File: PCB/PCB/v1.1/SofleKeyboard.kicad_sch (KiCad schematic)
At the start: 126 parts

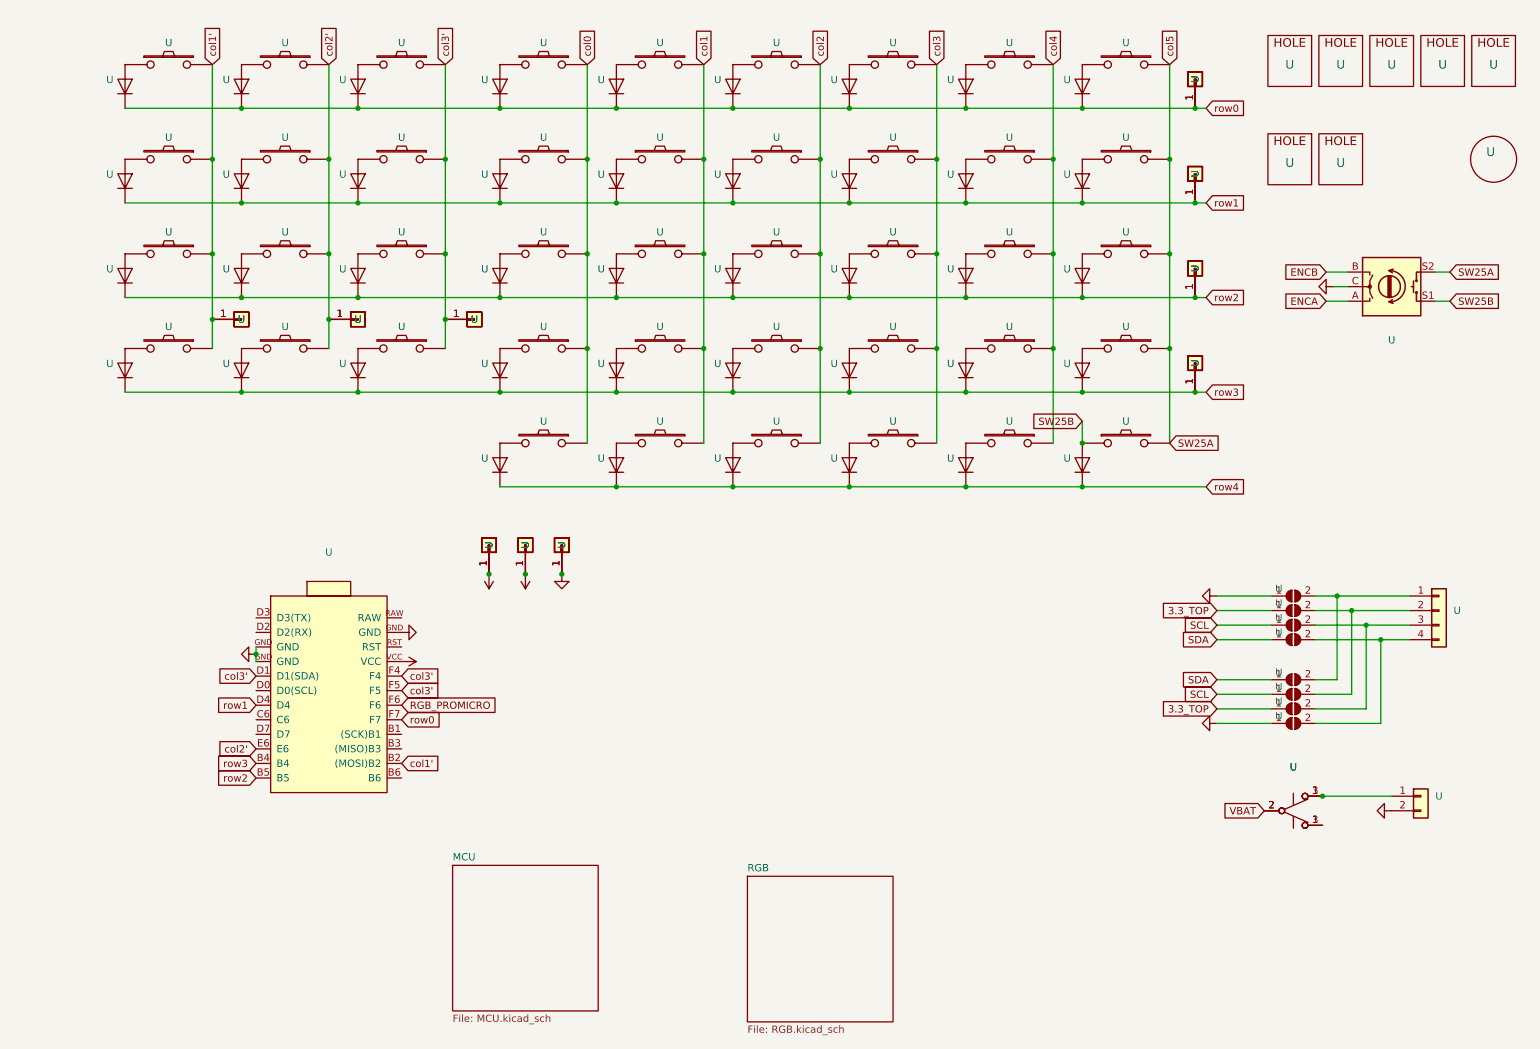
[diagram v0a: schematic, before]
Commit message: update PCB file
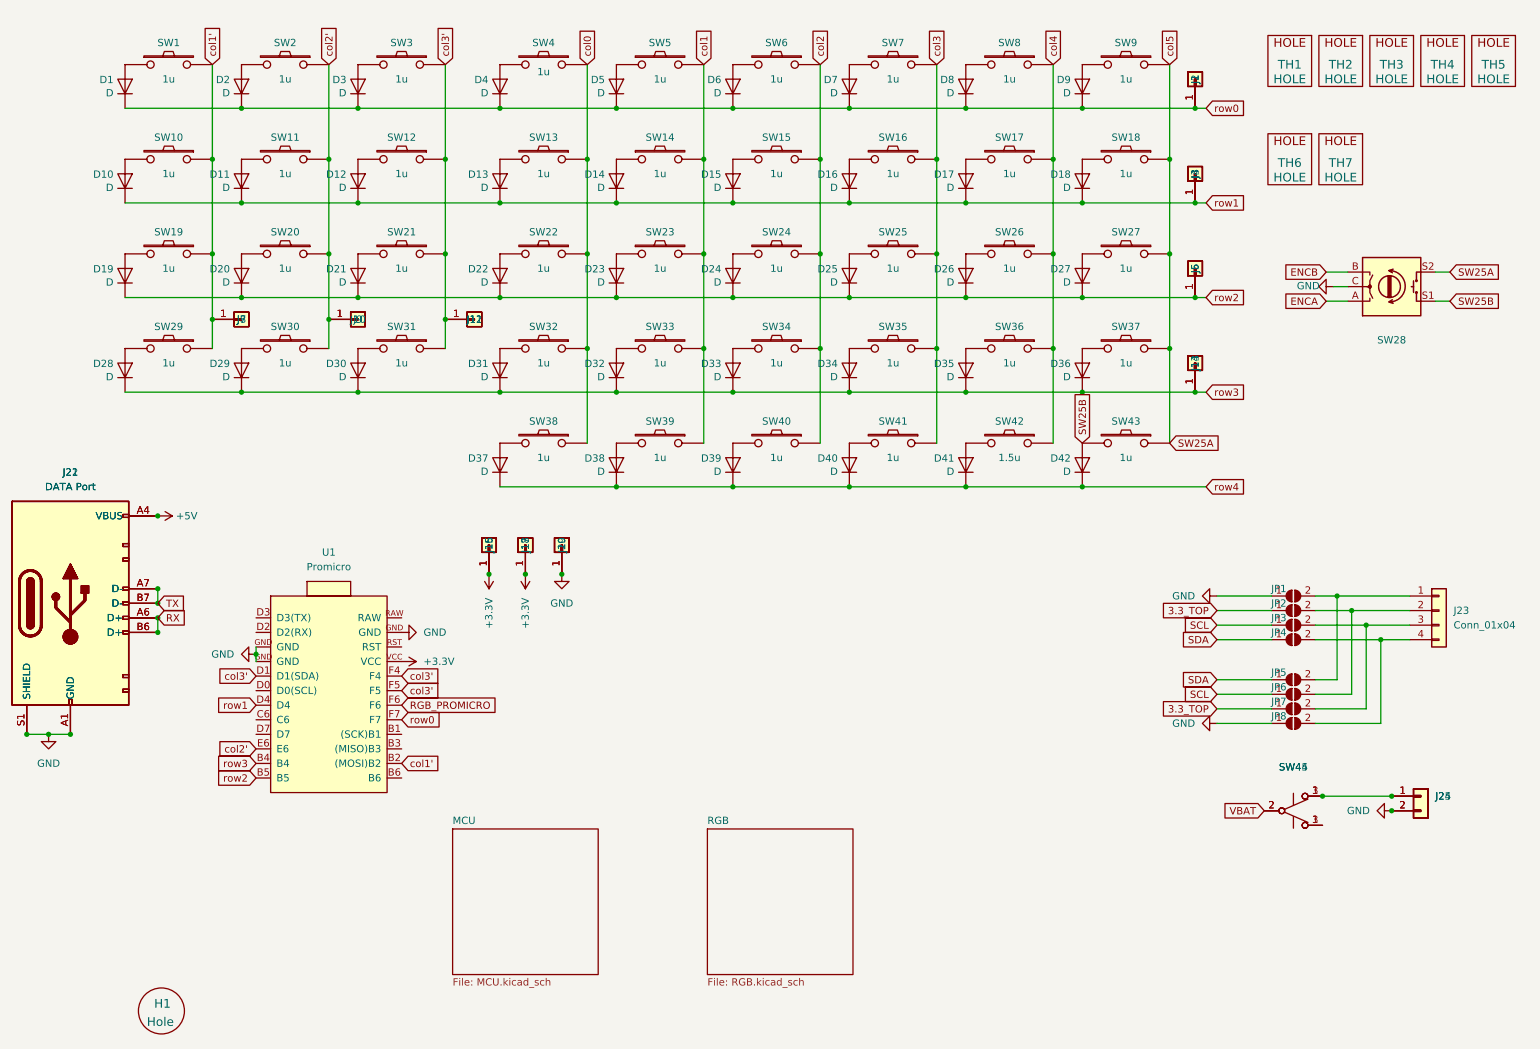
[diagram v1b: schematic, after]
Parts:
- removed U: (no value), symbol SofleKeyboard-rescue:SW_PUSH-Lily58-cache-Lily58_Pro-rescue
- added J21, J22: DATA Port, kien242:USB-C-16pin-hight-v2, symbol Connector:USB_C_Receptacle_USB2.0
- added J24: (no value), kien242:JST_PH_S2B-PH-SM4-TB_1x02-1MP_P2.00mm_Horizontal, symbol Connector_Generic:Conn_01x02
- added SW43: 1u, Library:SW-HS_flip-1u, symbol SofleKeyboard-rescue:SW_PUSH-Lily58-cache-Lily58_Pro-rescue
- D1, D10, D11, D12, D13, D14, D15, D16, D17, D18, D19, D2, D20, D21, D22, D23, D24, D25, D26, D27, D28, D29, D3, D30, D31, D32, D33, D34, D35, D36, D37, D38, D39, D4, D40, D41, D42, D5, D6, D7, D8, D9: renamed from U; value (none) -> D; footprint (none) -> Library:Diode
- H1: renamed from U; value (none) -> Hole; footprint (none) -> Library:Cut_hole
- J1, J10, J11, J12, J13, J14, J15, J16, J17, J18, J19, J2, J20, J3, J4, J5, J6, J7, J8, J9: renamed from U; value (none) -> (none); footprint (none) -> Library:Conn_01x01
- J23: renamed from U; value (none) -> Conn_01x04; footprint (none) -> kien242:128x64OLED
- J25: renamed from U; value (none) -> (none); footprint (none) -> kien242:JST_PH_S2B-PH-SM4-TB_1x02-1MP_P2.00mm_Horizontal
- JP1, JP2, JP3, JP4: renamed from U; value (none) -> (none); footprint (none) -> Jumper:SolderJumper-2_P1.3mm_Open_RoundedPad1.0x1.5mm
- JP5, JP6, JP7, JP8: renamed from U; value (none) -> (none); footprint (none) -> Jumper:SolderJumper-2_P1.3mm_Open_Pad1.0x1.5mm
- SW1, SW10, SW13, SW14, SW15, SW16, SW17, SW18, SW19, SW2, SW20, SW21, SW22, SW23, SW24, SW25, SW26, SW27, SW29, SW3, SW30, SW31, SW32, SW33, SW34, SW35, SW36, SW37, SW38, SW39, SW4, SW40, SW41, SW5, SW6, SW7, SW8, SW9: renamed from U; value (none) -> 1u; footprint (none) -> Library:SW-HS_flip-1u
- SW11, SW12: renamed from U; value (none) -> 1u; footprint (none) -> Library:SW-HS-Flip-1u
- SW28: renamed from U; value (none) -> (none); footprint (none) -> kien242:Econder
- SW42: renamed from U; value (none) -> 1.5u; footprint (none) -> Library:SW-HS_flip-1u
- SW44, SW45: renamed from U; value (none) -> (none); footprint (none) -> Button_Switch_SMD:SW_SPDT_PCM12
- TH1, TH2, TH3, TH4, TH5: renamed from U; value (none) -> HOLE; footprint (none) -> Library:HOLE_M2_TH
- TH6, TH7: renamed from U; value (none) -> HOLE; footprint (none) -> Library:M2_HOLE_PCB
- U1: renamed from U; value (none) -> Promicro; footprint (none) -> kien242:PRO-MICRO
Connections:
- net GND: now also J21.A1 (GND), J21.A12 (GND), J21.B1 (GND), J21.B12 (GND), J21.S1 (SHIELD), J22.A1 (GND), J22.A12 (GND), J22.B1 (GND), J22.B12 (GND), J22.S1 (SHIELD), J24.2 (Pin_2)
- net SW25A: now also SW43.1
- net SW25B: now also SW43.2
- net at J25.1 (Pin_1), SW44.1 (A), SW45.3 (C): now also J24.1 (Pin_1)
- new net +5V: J21.A4 (VBUS), J21.A9 (VBUS), J21.B4 (VBUS), J21.B9 (VBUS), J22.A4 (VBUS), J22.A9 (VBUS), J22.B4 (VBUS), J22.B9 (VBUS)
- new net RX: J21.A6 (D+), J21.B6 (D+), J22.A6 (D+), J22.B6 (D+)
- new net TX: J21.A7 (D-), J21.B7 (D-), J22.A7 (D-), J22.B7 (D-)
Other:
- moved on the sheet: H1
